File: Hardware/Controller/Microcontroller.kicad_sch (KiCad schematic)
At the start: 26 parts, among them J2 TagConnect_SWD, SW1 SW_Push, SW2 SW_Push, U1 W25Q64JVXGIQ, U3 RP2040, Y1 Crystal

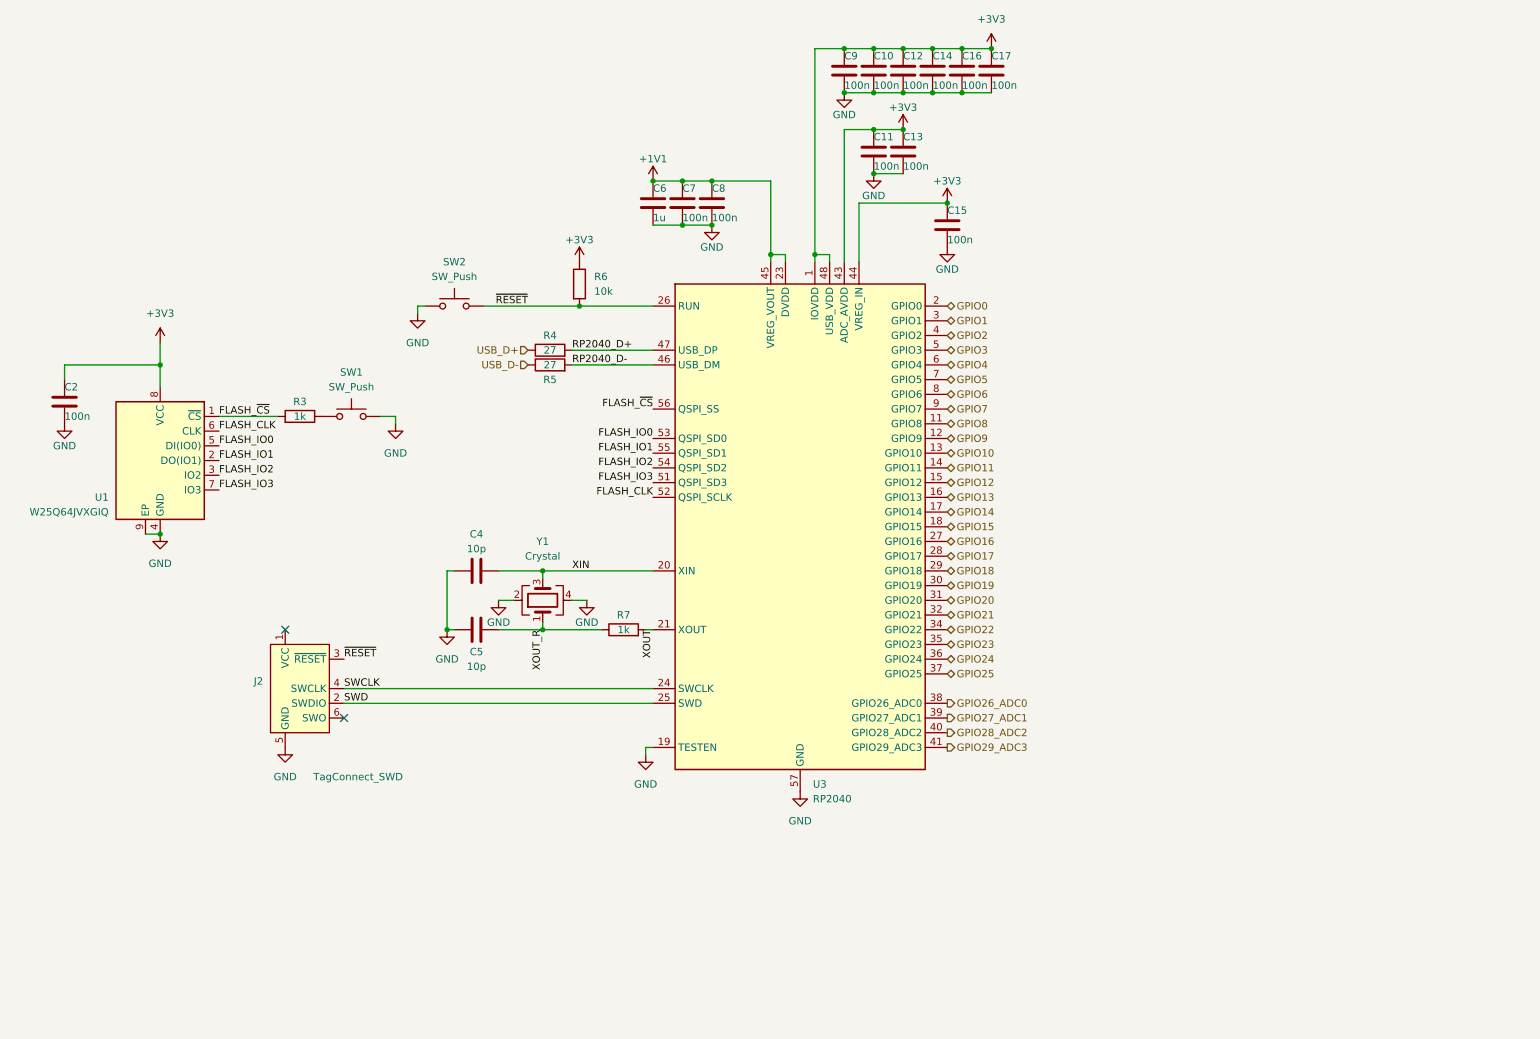
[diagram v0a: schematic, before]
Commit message: La in allt
Myyycket saker
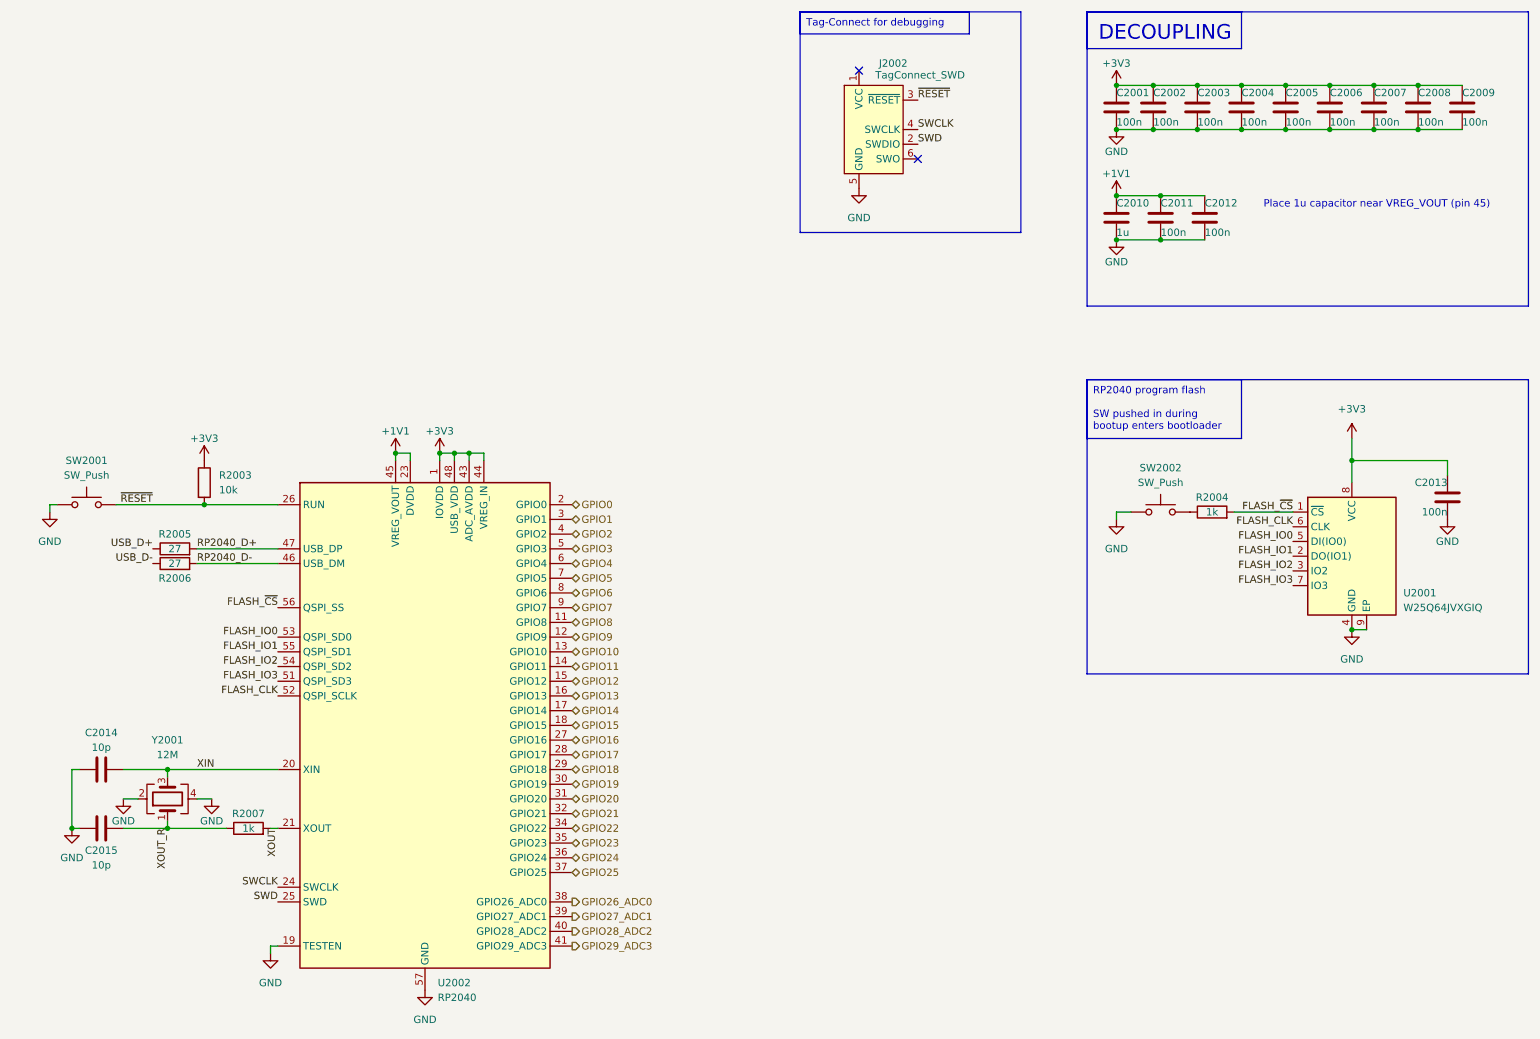
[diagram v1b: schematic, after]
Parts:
- removed C10, C11, C12, C13, C14, C15, C16, C17, C2, C7, C8, C9: 100n, Capacitor_SMD:C_0402_1005Metric, symbol Device:C
- removed C4, C5: 10p, Capacitor_SMD:C_0402_1005Metric, symbol Device:C
- removed C6: 1u, Capacitor_SMD:C_0402_1005Metric, symbol Device:C
- removed J2: TagConnect_SWD, Connector:Tag-Connect_TC2030-IDC-NL_2x03_P1.27mm_Vertical, symbol Connector:Conn_ARM_SWD_TagConnect_TC2030-NL
- removed R3, R7: 1k, Resistor_SMD:R_0402_1005Metric, symbol Device:R
- removed R4, R5: 27, Resistor_SMD:R_0402_1005Metric, symbol Device:R
- removed R6: 10k, Resistor_SMD:R_0402_1005Metric, symbol Device:R
- removed SW1, SW2: SW_Push, Button_Switch_SMD:SW_Push_SPST_NO_Alps_SKRK, symbol Switch:SW_Push
- removed U1: W25Q64JVXGIQ, Package_SON:WSON-8-1EP_4x4mm_P0.8mm_EP2.2x3mm, symbol Memory_Flash:W25Q32JVZP
- removed U3: RP2040, Package_DFN_QFN:QFN-56-1EP_7x7mm_P0.4mm_EP3.2x3.2mm, symbol MCU_RaspberryPi:RP2040
- removed Y1: Crystal, Crystal:Crystal_SMD_Abracon_ABM3B-4Pin_5.0x3.2mm, symbol Device:Crystal_GND24
- added C2001, C2002, C2003, C2004, C2005, C2006, C2007, C2008, C2009, C2011, C2012, C2013: 100n, Capacitor_SMD:C_0402_1005Metric, symbol Device:C
- added C2010: 1u, Capacitor_SMD:C_0402_1005Metric, symbol Device:C
- added C2014, C2015: 10p, Capacitor_SMD:C_0402_1005Metric, symbol Device:C
- added J2002: TagConnect_SWD, Connector:Tag-Connect_TC2030-IDC-NL_2x03_P1.27mm_Vertical, symbol Connector:Conn_ARM_SWD_TagConnect_TC2030-NL
- added R2003: 10k, Resistor_SMD:R_0402_1005Metric, symbol Device:R
- added R2004, R2007: 1k, Resistor_SMD:R_0402_1005Metric, symbol Device:R
- added R2005, R2006: 27, Resistor_SMD:R_0402_1005Metric, symbol Device:R
- added SW2001, SW2002: SW_Push, Button_Switch_SMD:SW_Push_SPST_NO_Alps_SKRK, symbol Switch:SW_Push
- added U2001: W25Q64JVXGIQ, Package_SON:WSON-8-1EP_4x4mm_P0.8mm_EP2.2x3mm, symbol Memory_Flash:W25Q32JVZP
- added U2002: RP2040, Package_DFN_QFN:QFN-56-1EP_7x7mm_P0.4mm_EP3.2x3.2mm, symbol MCU_RaspberryPi:RP2040
- added Y2001: 12M, Crystal:Crystal_SMD_Abracon_ABM3B-4Pin_5.0x3.2mm, symbol Device:Crystal_GND24
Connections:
- net +1V1: now also C2010.1, C2011.1, C2012.1, U2002.23 (DVDD), U2002.45 (VREG_VOUT), U2002.50 (DVDD)
- net +3V3: now also C2001.1, C2002.1, C2003.1, C2004.1, C2005.1, C2006.1, C2007.1, C2008.1, C2009.1, C2013.1, R2003.1, U2001.8 (VCC), U2002.1 (IOVDD), U2002.10 (IOVDD), U2002.22 (IOVDD), U2002.33 (IOVDD), U2002.42 (IOVDD), U2002.43 (ADC_AVDD), U2002.44 (VREG_IN), U2002.48 (USB_VDD), U2002.49 (IOVDD)
- net FLASH_CLK: now also U2001.6 (CLK), U2002.52 (QSPI_SCLK)
- net FLASH_IO0: now also U2001.5 (DI(IO0)), U2002.53 (QSPI_SD0)
- net FLASH_IO1: now also U2001.2 (DO(IO1)), U2002.55 (QSPI_SD1)
- net FLASH_IO2: now also U2001.3 (IO2), U2002.54 (QSPI_SD2)
- net FLASH_IO3: now also U2001.7 (IO3), U2002.51 (QSPI_SD3)
- net FLASH_~{CS}: now also R2004.2, U2001.1 (~{CS}), U2002.56 (QSPI_SS)
- net GND: now also C2001.2, C2002.2, C2003.2, C2004.2, C2005.2, C2006.2, C2007.2, C2008.2, C2009.2, C2010.2, C2011.2, C2012.2, C2013.2, C2014.1, C2015.1, J2002.5 (GND), SW2001.2, SW2002.1, U2001.4 (GND), U2001.9 (EP), U2002.19 (TESTEN), U2002.57 (GND), Y2001.2, Y2001.4
- net GPIO0: now also U2002.2 (GPIO0)
- net GPIO1: now also U2002.3 (GPIO1)
- net GPIO10: now also U2002.13 (GPIO10)
- net GPIO11: now also U2002.14 (GPIO11)
- net GPIO12: now also U2002.15 (GPIO12)
- net GPIO13: now also U2002.16 (GPIO13)
- net GPIO14: now also U2002.17 (GPIO14)
- net GPIO15: now also U2002.18 (GPIO15)
- net GPIO16: now also U2002.27 (GPIO16)
- net GPIO17: now also U2002.28 (GPIO17)
- net GPIO18: now also U2002.29 (GPIO18)
- net GPIO19: now also U2002.30 (GPIO19)
- net GPIO2: now also U2002.4 (GPIO2)
- net GPIO20: now also U2002.31 (GPIO20)
- net GPIO21: now also U2002.32 (GPIO21)
- net GPIO22: now also U2002.34 (GPIO22)
- net GPIO23: now also U2002.35 (GPIO23)
- net GPIO24: now also U2002.36 (GPIO24)
- net GPIO25: now also U2002.37 (GPIO25)
- net GPIO26_ADC0: now also U2002.38 (GPIO26_ADC0)
- net GPIO27_ADC1: now also U2002.39 (GPIO27_ADC1)
- net GPIO28_ADC2: now also U2002.40 (GPIO28_ADC2)
- net GPIO29_ADC3: now also U2002.41 (GPIO29_ADC3)
- net GPIO3: now also U2002.5 (GPIO3)
- net GPIO4: now also U2002.6 (GPIO4)
- net GPIO5: now also U2002.7 (GPIO5)
- net GPIO6: now also U2002.8 (GPIO6)
- net GPIO7: now also U2002.9 (GPIO7)
- net GPIO8: now also U2002.11 (GPIO8)
- net GPIO9: now also U2002.12 (GPIO9)
- net RP2040_D+: now also R2005.2, U2002.47 (USB_DP)
- net RP2040_D-: now also R2006.2, U2002.46 (USB_DM)
- net SWCLK: now also J2002.4 (SWCLK), U2002.24 (SWCLK)
- net SWD: now also J2002.2 (SWDIO), U2002.25 (SWD)
- net USB_D+: now also R2005.1
- net USB_D-: now also R2006.1
- net XIN: now also C2014.2, U2002.20 (XIN), Y2001.3
- net XOUT: now also R2007.2, U2002.21 (XOUT)
- net XOUT_R: now also C2015.2, R2007.1, Y2001.1
- net ~{RESET}: now also J2002.3 (~{RESET}), R2003.2, SW2001.1, U2002.26 (RUN)
- new net: R2004.1, SW2002.2
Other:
- note added: "Place 1u capacitor near VREG_VOUT (pin 45)"
